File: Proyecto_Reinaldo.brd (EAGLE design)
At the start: 60 x 40 mm, 43 parts, among them IC2 MC34063A, U1 ATMEGA328P-AU

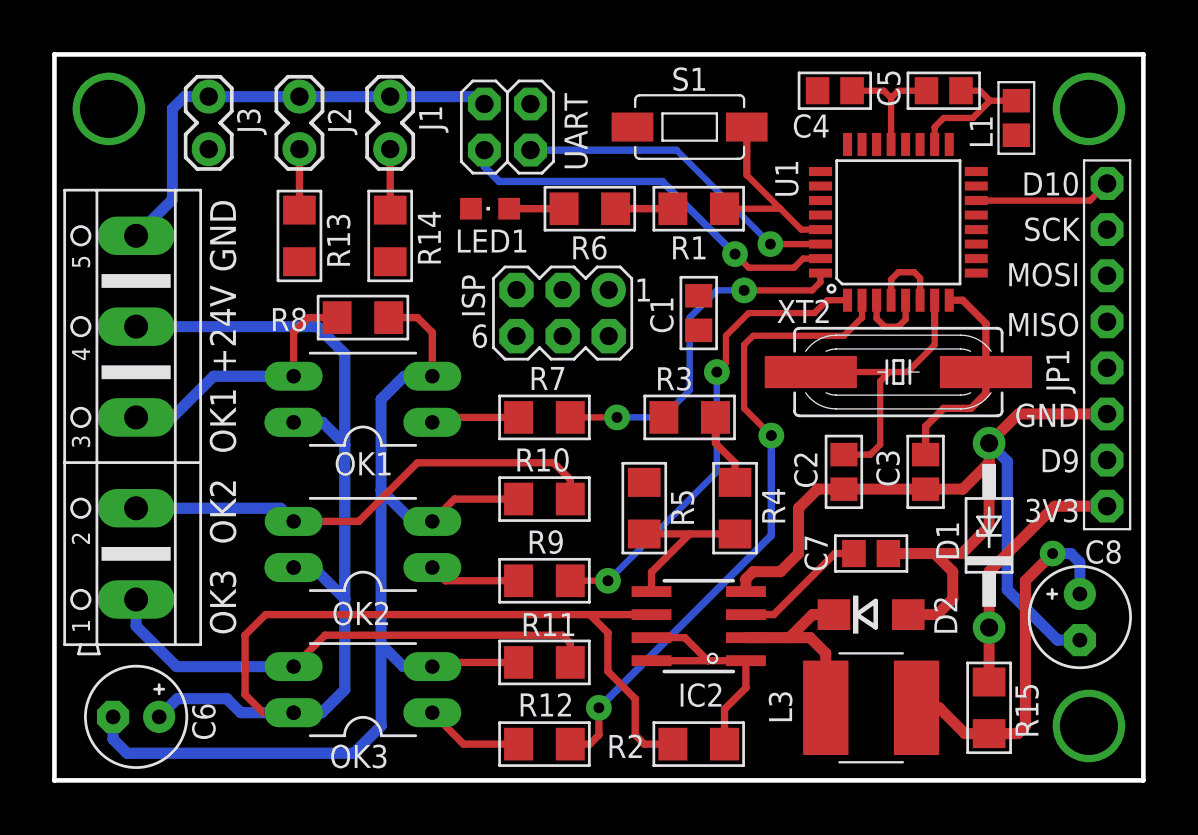
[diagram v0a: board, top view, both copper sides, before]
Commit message: Terminado BRD, inicio revision
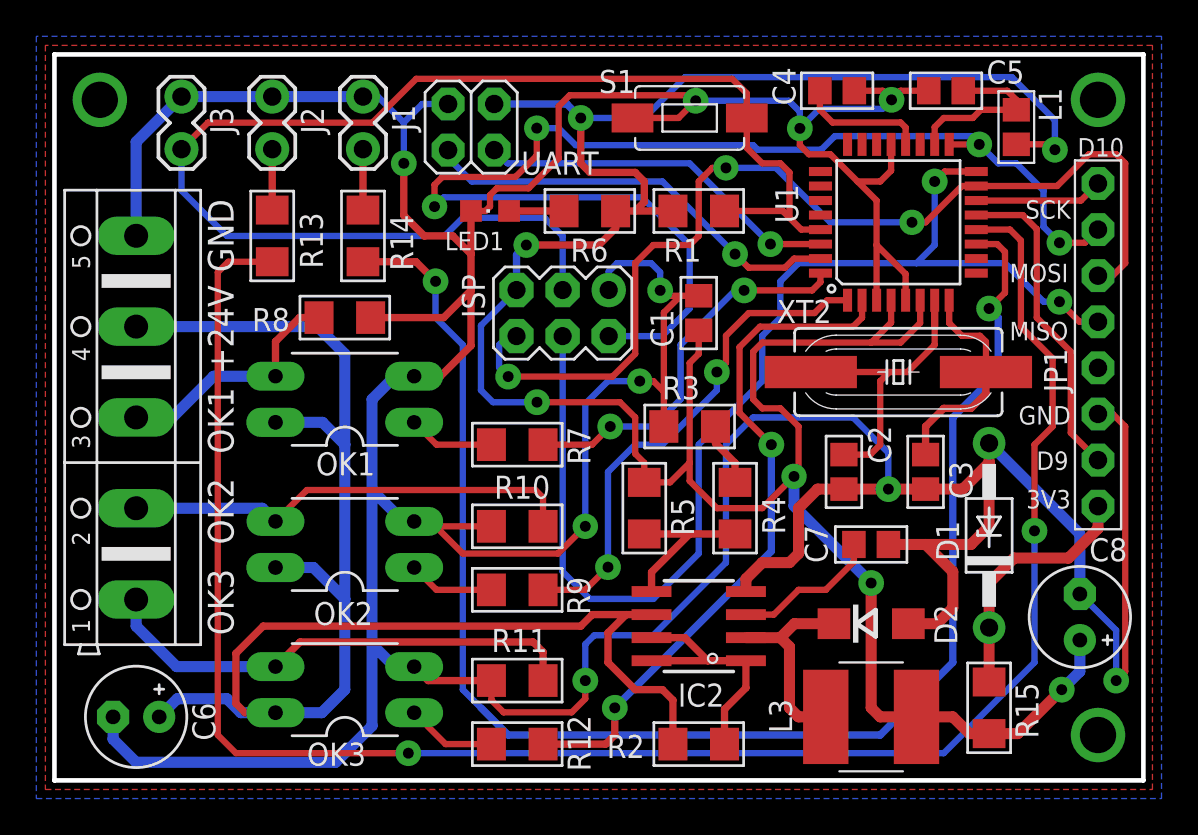
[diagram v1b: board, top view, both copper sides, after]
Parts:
- moved U$1 13.2 mm to (38.0, 6.50)
- moved R10 2.12 mm to (25.5, 14.0)
- moved R7 2.12 mm to (25.5, 18.5)
- moved UART 2.00 mm to (25.5, 36.0)
- moved R11 1.80 mm to (25.5, 5.50)
- moved R9 1.58 mm to (25.5, 10.5)
- moved J1 1.50 mm to (17.0, 37.5)
- moved J2 1.50 mm to (12.0, 37.5)
- moved J3 1.50 mm to (7.00, 37.5)
- moved R12 1.50 mm to (25.5, 2.00)
- moved R13 1.50 mm to (12.0, 30.0)
- moved R14 1.50 mm to (17.0, 30.0)
- moved OK1 1.00 mm to (16.0, 21.0)
- moved OK2 1.00 mm to (16.0, 13.0)
- moved OK3 1.00 mm to (16.0, 5.00)
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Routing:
- net GND: track 152.4 -> 303.8 mm, vias 0 -> 10
- net VCC: track 27.7 -> 147.4 mm, vias 1 -> 7
- net D8: track 0.00 -> 103.3 mm, vias 0 -> 2
- net D7: track 0.00 -> 83.2 mm, vias 0 -> 2
- net SCK: track 0.00 -> 70.2 mm, vias 0 -> 4
- net MISO: track 0.00 -> 65.7 mm, vias 0 -> 2
- net RST: track 11.0 -> 75.3 mm
- net MOSI: track 0.00 -> 56.9 mm, vias 0 -> 3
- net D9: track 0.00 -> 17.8 mm
- net AREF: track 0.00 -> 7.11 mm
- net D4: track 35.9 -> 38.2 mm
- net D3: track 25.8 -> 27.9 mm
- net RX0: track 18.1 -> 20.1 mm
- net OK2: track 27.0 -> 25.2 mm
- net TX1: track 21.9 -> 23.7 mm
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- added copper zone on layer 1, net GND
- added copper zone on layer 16, net GND
